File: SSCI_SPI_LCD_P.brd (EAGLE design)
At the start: 110 x 100 mm, 123 parts, among them IC13 74LVC541_RGY, IC18 74LVC541_RGY, IC3 74LVC541_RGY, IC8 74LVC541_RGY, X1 PHA-1X08SG, X2 PHA-1X08SG, X3 PHA-1X08SG, X4 PHA-1X08SG, X5 PHA-1X08SG, X6 PHA-1X08SG, X7 PHA-1X08SG, X8 PHA-1X08SG

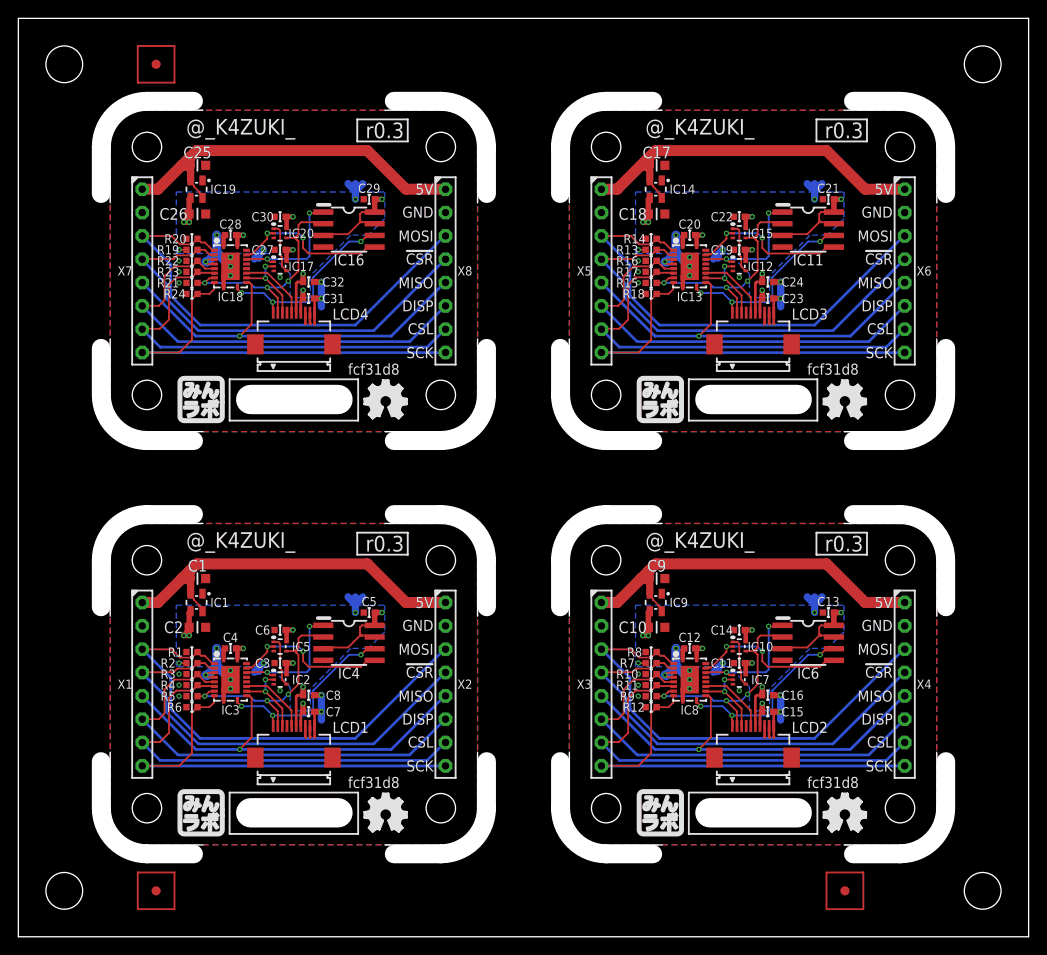
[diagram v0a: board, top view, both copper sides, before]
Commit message: 8c37b00 panelized
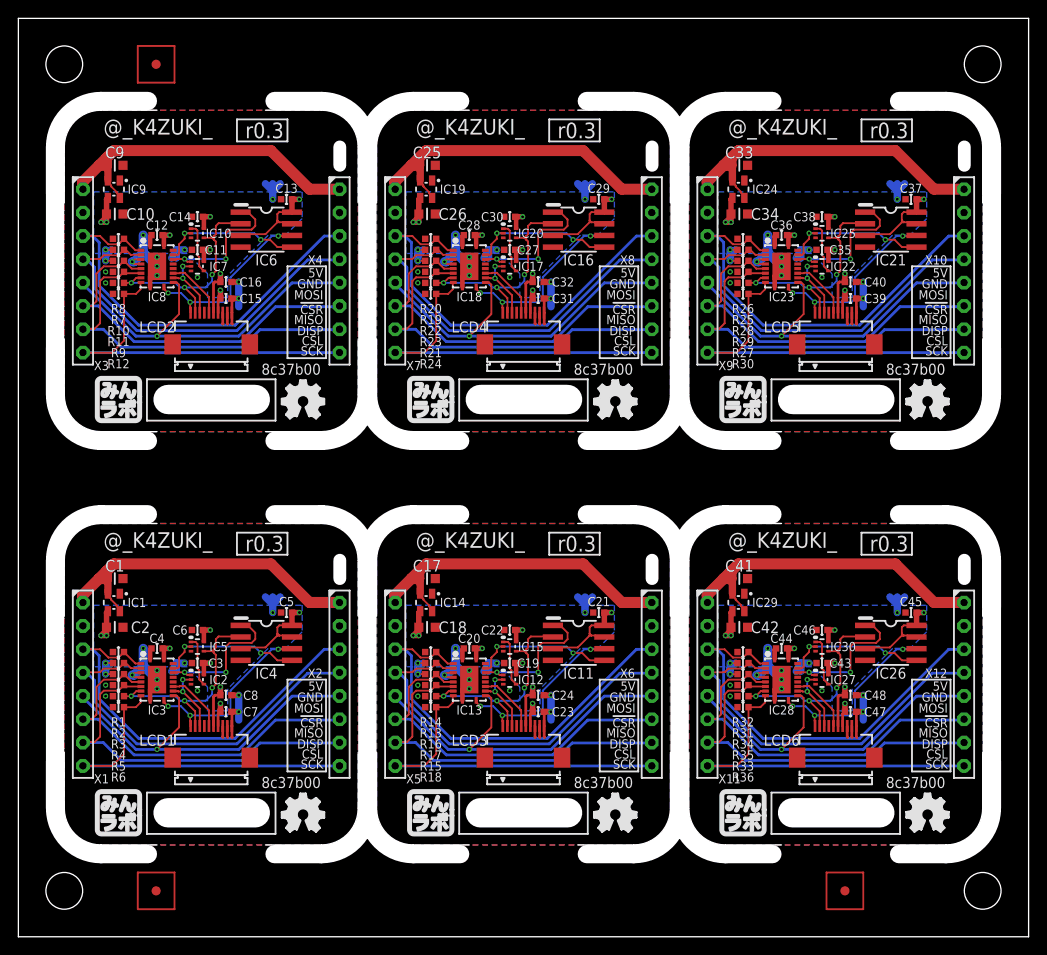
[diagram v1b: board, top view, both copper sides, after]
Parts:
- added C33, C34, C41, C42: (no value), mylib:CR_1608
- added C35, C36, C37, C38, C39, C40, C43, C44, C45, C46, C47, C48, R25, R26, R27, R28, R29, R30, R31, R32, R33, R34, R35, R36: (no value), mylib:C0402
- added GIT5, GIT6: 8c37b00, git-revision:GIT-REVISION_1.2
- added I5, I6: (no value), mylib:ICON_MINLAB_5.2MM
- added IC21, IC26: (no value), mylib:IC_08_1.27_150MIL
- added IC22, IC25, IC27, IC30: (no value), mylib:SOT50P160X120-5N
- added IC23, IC28: 74LVC541_RGY, mylib:QFN50P460X360-20N
- added IC24, IC29: (no value), mylib:SOT130P220X135-4N
- added ICON10, ICON12: (no value), mylib:ICON_OSHW
- added ICON11, ICON9: r0.3, mylib:ICON_REVISION1.7
- added LCD5, LCD6: LCD_GLCD_400X240, mylib:LCD_GLCD_400X240
- added P17, P18, P19, P20, P21, P22, P23, P24: (no value), mylib:PCB_CORNER_NH
- added X10, X11, X12, X9: PHA-1X08SG, mylib:PHA-1X08SG
- GIT1, GIT2, GIT3, GIT4: value fcf31d8 -> 8c37b00
- P1, P10, P11, P12, P13, P14, P15, P16, P2, P3, P4, P5, P6, P7, P8, P9: device mylib:PCB_CORNER -> mylib:PCB_CORNER_NH
- moved ICON3 77.5 mm to (26.9, 87.8)
- moved P5 77.4 mm to (33.0, 59.0)
- moved P6 77.4 mm to (33.0, 86.0)
- moved X4 76.2 mm to (35.0, 72.5)
- moved C10 74.2 mm to (10.5, 78.7)
- moved C11 74.2 mm to (19.5, 74.8)
- moved C13 74.2 mm to (29.2, 80.3)
- moved C14 74.2 mm to (19.5, 78.4)
- moved C9 74.2 mm to (10.5, 84.0)
- moved GIT2 74.2 mm to (29.7, 61.8)
- moved IC6 74.2 mm to (27.0, 77.0)
- moved IC7 74.2 mm to (19.5, 73.0)
- moved IC9 74.2 mm to (10.4, 81.4)
- moved ICON4 74.2 mm to (31.0, 58.3)
- moved LCD2 74.2 mm to (21.0, 64.5)
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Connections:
- new net !CSR!-4: IC21.1, IC22.1, IC23.17
- new net !CSR!-5: IC26.1, IC27.1, IC28.17
- new net !CSR!4: IC23.3, R25.2, X10.4, X9.4
- new net !CSR!5: IC28.3, R31.2, X11.4, X12.4
- new net 3.3V4: C34.1, C35.1, C36.1, C37.1, C38.1, C39.1, C40.1, IC21.3, IC21.7, IC21.8, IC22.5, IC23.20, IC24.3, IC25.5, LCD5.6, LCD5.7, R25.1, R28.1
- new net 3.3V5: C42.1, C43.1, C44.1, C45.1, C46.1, C47.1, C48.1, IC26.3, IC26.7, IC26.8, IC27.5, IC28.20, IC29.3, IC30.5, LCD6.6, LCD6.7, R31.1, R34.1
- new net 5V4: C33.1, IC24.2, IC24.4, X10.1, X9.1
- new net 5V5: C41.1, IC29.2, IC29.4, X11.1, X12.1
- new net CSL-4: IC22.2, IC23.13, LCD5.3
- new net CSL-5: IC27.2, IC28.13, LCD6.3
- new net CSL4: IC23.7, R29.2, X10.7, X9.7
- new net CSL5: IC28.7, R35.2, X11.7, X12.7
- new net DISP-4: IC23.14, LCD5.5
- new net DISP-5: IC28.14, LCD6.5
- new net DISP4: IC23.6, R28.2, X10.6, X9.6
- new net DISP5: IC28.6, R34.2, X11.6, X12.6
- new net GND4: C33.2, C34.2, C35.2, C36.2, C37.2, C38.2, C39.2, C40.2, IC21.4, IC22.3, IC23.1, IC23.10, IC23.19, IC23.4, IC23.5, IC23.EP, IC24.1, IC25.3, LCD5.10, LCD5.8, LCD5.9, LCD5.PAD1, LCD5.PAD2, R26.1, R27.1, R29.1, R30.1, X10.2, X9.2
- new net GND5: C41.2, C42.2, C43.2, C44.2, C45.2, C46.2, C47.2, C48.2, IC26.4, IC27.3, IC28.1, IC28.10, IC28.19, IC28.4, IC28.5, IC28.EP, IC29.1, IC30.3, LCD6.10, LCD6.8, LCD6.9, LCD6.PAD1, LCD6.PAD2, R32.1, R33.1, R35.1, R36.1, X11.2, X12.2
- new net MISO-4: IC21.2, IC23.8, IC25.4, LCD5.2, R27.2
- new net MISO-5: IC26.2, IC28.8, IC30.4, LCD6.2, R33.2
- new net MISO4: IC23.12, X10.5, X9.5
- new net MISO5: IC28.12, X11.5, X12.5
- new net MOSI-4: IC21.5, IC23.18, IC25.2
- new net MOSI-5: IC26.5, IC28.18, IC30.2
- new net MOSI4: IC23.2, R26.2, X10.3, X9.3
- new net MOSI5: IC28.2, R32.2, X11.3, X12.3
- new net N$5: IC22.4, IC25.1
- new net N$6: IC27.4, IC30.1
- new net SCK-4: IC21.6, IC23.11, LCD5.1
- new net SCK-5: IC26.6, IC28.11, LCD6.1
- new net SCK4: IC23.9, R30.2, X10.8, X9.8
- new net SCK5: IC28.9, R36.2, X11.8, X12.8
- net 3.3V: now also R3.1
- net 3.3V1: now also R10.1
- net 3.3V2: now also R16.1
- net 3.3V3: now also R22.1
- net GND: no longer R3.1
- net GND1: no longer R10.1
- net GND2: no longer R16.1
- net GND3: no longer R22.1
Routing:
- net MOSI5: track 0.00 -> 46.3 mm
- net MOSI4: track 0.00 -> 46.3 mm
- net !CSR!5: track 0.00 -> 42.9 mm
- net !CSR!4: track 0.00 -> 42.9 mm
- net DISP5: track 0.00 -> 41.7 mm
- net DISP4: track 0.00 -> 41.7 mm
- net CSL4: track 0.00 -> 41.3 mm
- net CSL5: track 0.00 -> 41.3 mm
- net SCK5: track 0.00 -> 40.9 mm
- net SCK4: track 0.00 -> 40.9 mm
- net MISO5: track 0.00 -> 40.3 mm, vias 0 -> 1
- net MISO4: track 0.00 -> 40.3 mm, vias 0 -> 1
- net 5V5: track 0.00 -> 38.9 mm
- net 5V4: track 0.00 -> 38.9 mm
- net 3.3V4: track 0.00 -> 32.9 mm, vias 0 -> 10
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- added copper zone on layer 16, net 3.3V4
- added copper zone on layer 16, net 3.3V5
- added copper zone on layer 1, net GND4
- added copper zone on layer 16, net GND4
- added copper zone on layer 1, net GND5
- added copper zone on layer 16, net GND5
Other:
- outline, holes or cut-outs redrawn
